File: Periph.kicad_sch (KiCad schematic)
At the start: 17 parts, among them J4 SM04B-GHS-TB, U10 ICM-42688-P, U11 BMP388, U9 W25Q128JVSIQ

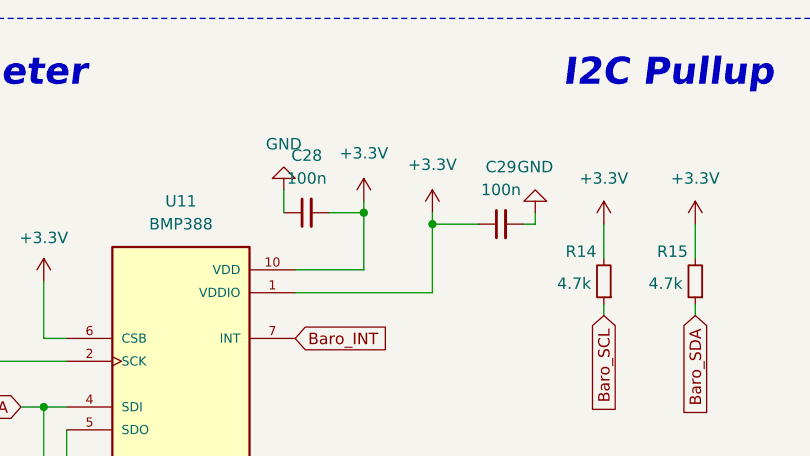
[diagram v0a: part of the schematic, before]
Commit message: PumbaaV2_RC2
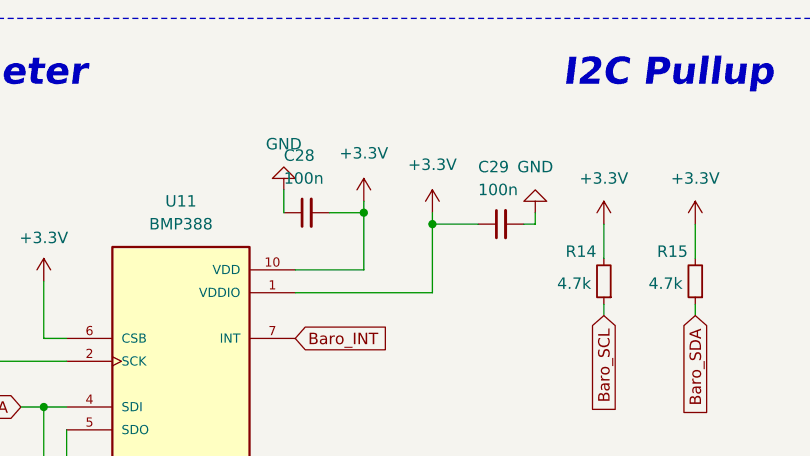
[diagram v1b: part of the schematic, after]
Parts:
- C28, C29: footprint Capacitor_SMD:C_0201_0603Metric -> Capacitor_SMD:C_0402_1005Metric; LCSC Part # (none) -> C1525
- J4: value SM04B-GHS-TB -> SM04B-GHS-TB(LF)(SN)
- LSE1: LCSC Part  C2650753 -> C2650753 C5280579
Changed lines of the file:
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@@
-	(symbol
-		(lib_id "Device:C_Small")
-		(at 215.9 45.72 90)
-		(unit 1)
-		(exclude_from_sim no)
-		(in_bom yes)
-		(on_board yes)
-		(dnp no)
-		(fields_autoplaced yes)
-		(property "Reference" "C28"
-			(at 215.9063 39.37 90)
-			(effects
-				(font
-					(size 1.27 1.27)
-				)
-			)
-		)
-		(property "Value" "100n"
-			(at 215.9063 41.91 90)
-			(effects
-				(font
-					(size 1.27 1.27)
-				)
-			)
-		)
-		(property "Footprint" "Capacitor_SMD:C_0201_0603Metric"
-			(at 215.9 45.72 0)
-			(effects
-				(font
-					(size 1.27 1.27)
-				)
-				(hide yes)
-			)
-		)
-		(property "Datasheet" "~"
-			(at 215.9 45.72 0)
-			(effects
-				(font
-					(size 1.27 1.27)
-				)
-				(hide yes)
-			)
-		)
-		(property "Description" ""
-			(at 215.9 45.72 0)
-			(effects
-				(font
-					(size 1.27 1.27)
-				)
-			)
-		)
-		(pin "1"
-		)
-		(pin "2"
-		)
-		(instances
-			(project "MX_IMU"
-				(path "/8ed38441-7d4e-4e89-870f-07e11c6dce38/57f4b5bf-da86-4b65-9b05-7c9ef99c472c"
-					(reference "C28")
-					(unit 1)
-				)
-			)
-		)
-	)
 	(symbol
 		(lib_id "Device:C_Small")
@@
 			)
 		)
-		(property "Value" "SM04B-GHS-TB"
+		(property "Value" "SM04B-GHS-TB(LF)(SN)"
 			(at 209.55 91.4399 0)
 			(effects
@@
 	)
 	(symbol
+		(lib_id "Device:C_Small")
+		(at 237.49 46.99 90)
+		(unit 1)
+		(exclude_from_sim no)
+		(in_bom yes)
+		(on_board yes)
+		(dnp no)
+		(property "Reference" "C29"
+			(at 234.95 40.64 90)
+			(effects
+				(font
+					(size 1.27 1.27)
+				)
+				(justify right)
+			)
+		)
+		(property "Value" "100n"
+			(at 234.95 43.18 90)
+			(effects
+				(font
+					(size 1.27 1.27)
+				)
+				(justify right)
+			)
+		)
+		(property "Footprint" "Capacitor_SMD:C_0402_1005Metric"
+			(at 237.49 46.99 0)
+			(effects
+				(font
+					(size 1.27 1.27)
+				)
+				(hide yes)
+			)
+		)
+		(property "Datasheet" "~"
+			(at 237.49 46.99 0)
+			(effects
+				(font
+					(size 1.27 1.27)
+				)
+				(hide yes)
+			)
+		)
+		(property "Description" ""
+			(at 237.49 46.99 0)
+			(effects
+				(font
+					(size 1.27 1.27)
+				)
+			)
+		)
+		(property "LCSC Part #" "C1525"
+			(at 237.49 46.99 0)
+			(effects
+				(font
+					(size 1.27 1.27)
+				)
+				(hide yes)
+			)
+		)
+		(pin "2"
+		)
+		(pin "1"
+		)
+		(instances
+			(project "MX_IMU"
+				(path "/8ed38441-7d4e-4e89-870f-07e11c6dce38/57f4b5bf-da86-4b65-9b05-7c9ef99c472c"
+					(reference "C29")
+					(unit 1)
+				)
+			)
+		)
+	)
+	(symbol
 		(lib_id "power:+3.3V")
 		(at 186.69 53.34 0)
@@
 			)
 		)
-		(property "LCSC Part " "C2650753"
+		(property "LCSC Part " "C2650753  C5280579"
 			(at 82.55 38.1 0)
 			(effects
@@
 				(path "/8ed38441-7d4e-4e89-870f-07e11c6dce38/57f4b5bf-da86-4b65-9b05-7c9ef99c472c"
 					(reference "LSE1")
-					(unit 1)
-				)
-			)
-		)
-	)
-	(symbol
-		(lib_id "Device:C_Small")
-		(at 237.49 46.99 90)
-		(unit 1)
-		(exclude_from_sim no)
-		(in_bom yes)
-		(on_board yes)
-		(dnp no)
-		(fields_autoplaced yes)
-		(property "Reference" "C29"
-			(at 237.4963 40.64 90)
-			(effects
-				(font
-					(size 1.27 1.27)
-				)
-			)
-		)
-		(property "Value" "100n"
-			(at 237.4963 43.18 90)
-			(effects
-				(font
-					(size 1.27 1.27)
-				)
-			)
-		)
-		(property "Footprint" "Capacitor_SMD:C_0201_0603Metric"
-			(at 237.49 46.99 0)
-			(effects
-				(font
-					(size 1.27 1.27)
-				)
-				(hide yes)
-			)
-		)
-		(property "Datasheet" "~"
-			(at 237.49 46.99 0)
-			(effects
-				(font
-					(size 1.27 1.27)
-				)
-				(hide yes)
-			)
-		)
-		(property "Description" ""
-			(at 237.49 46.99 0)
-			(effects
-				(font
-					(size 1.27 1.27)
-				)
-			)
-		)
-		(pin "1"
-		)
-		(pin "2"
-		)
-		(instances
-			(project "MX_IMU"
-				(path "/8ed38441-7d4e-4e89-870f-07e11c6dce38/57f4b5bf-da86-4b65-9b05-7c9ef99c472c"
-					(reference "C29")
 					(unit 1)
 				)
@@
 					(unit 1)
 				)
+			)
+		)
+	)
+	(symbol
+		(lib_id "Device:C_Small")
+		(at 215.9 45.72 90)
+		(unit 1)
+		(exclude_from_sim no)
+		(in_bom yes)
+		(on_board yes)
+		(dnp no)
+		(property "Reference" "C28"
+			(at 213.36 39.37 90)
+			(effects
+				(font
+					(size 1.27 1.27)
+				)
+				(justify right)
+			)
+		)
+		(property "Value" "100n"
+			(at 213.36 41.91 90)
+			(effects
+				(font
+					(size 1.27 1.27)
+				)
+				(justify right)
+			)
+		)
+		(property "Footprint" "Capacitor_SMD:C_0402_1005Metric"
+			(at 215.9 45.72 0)
+			(effects
+				(font
+					(size 1.27 1.27)
+				)
+				(hide yes)
+			)
+		)
+		(property "Datasheet" "~"
+			(at 215.9 45.72 0)
+			(effects
+				(font
+					(size 1.27 1.27)
+				)
+				(hide yes)
+			)
+		)
+		(property "Description" ""
+			(at 215.9 45.72 0)
+			(effects
+				(font
+					(size 1.27 1.27)
+				)
+			)
+		)
+		(property "LCSC Part #" "C1525"
+			(at 215.9 45.72 0)
+			(effects
+				(font
+					(size 1.27 1.27)
+				)
+				(hide yes)
+			)
+		)
+		(pin "2"
+		)
+		(pin "1"
+		)
+		(instances
+			(project "MX_IMU"
+				(path "/8ed38441-7d4e-4e89-870f-07e11c6dce38/57f4b5bf-da86-4b65-9b05-7c9ef99c472c"
+					(reference "C28")
+					(unit 1)
+				)
